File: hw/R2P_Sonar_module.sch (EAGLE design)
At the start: 36 parts, among them U1 STM32F103CX, U5 LD3985XX, X1 MICROMATCH-4, X2 MICROMATCH-6, X3 MICROMATCH-6-SIDE

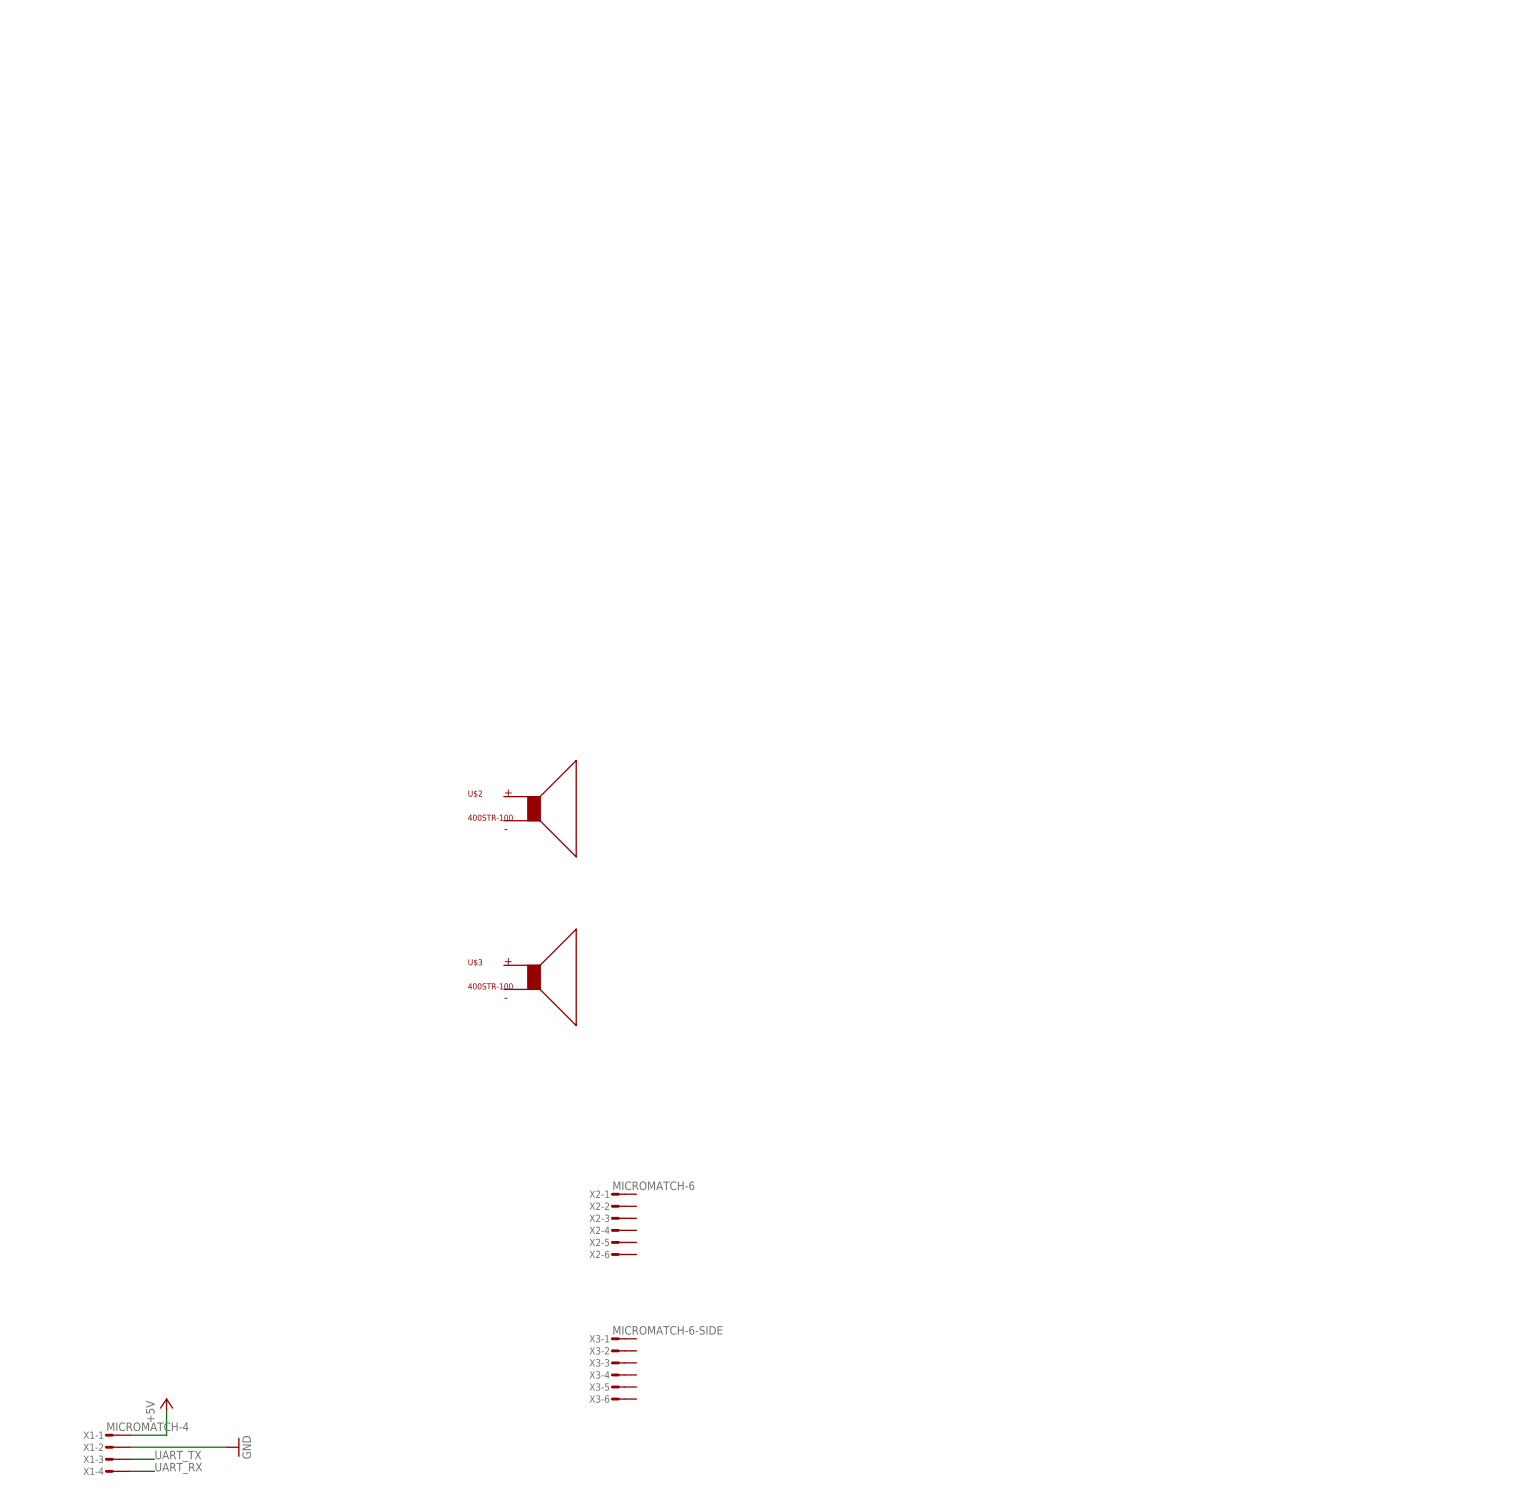
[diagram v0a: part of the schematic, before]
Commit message: Ongoing layout
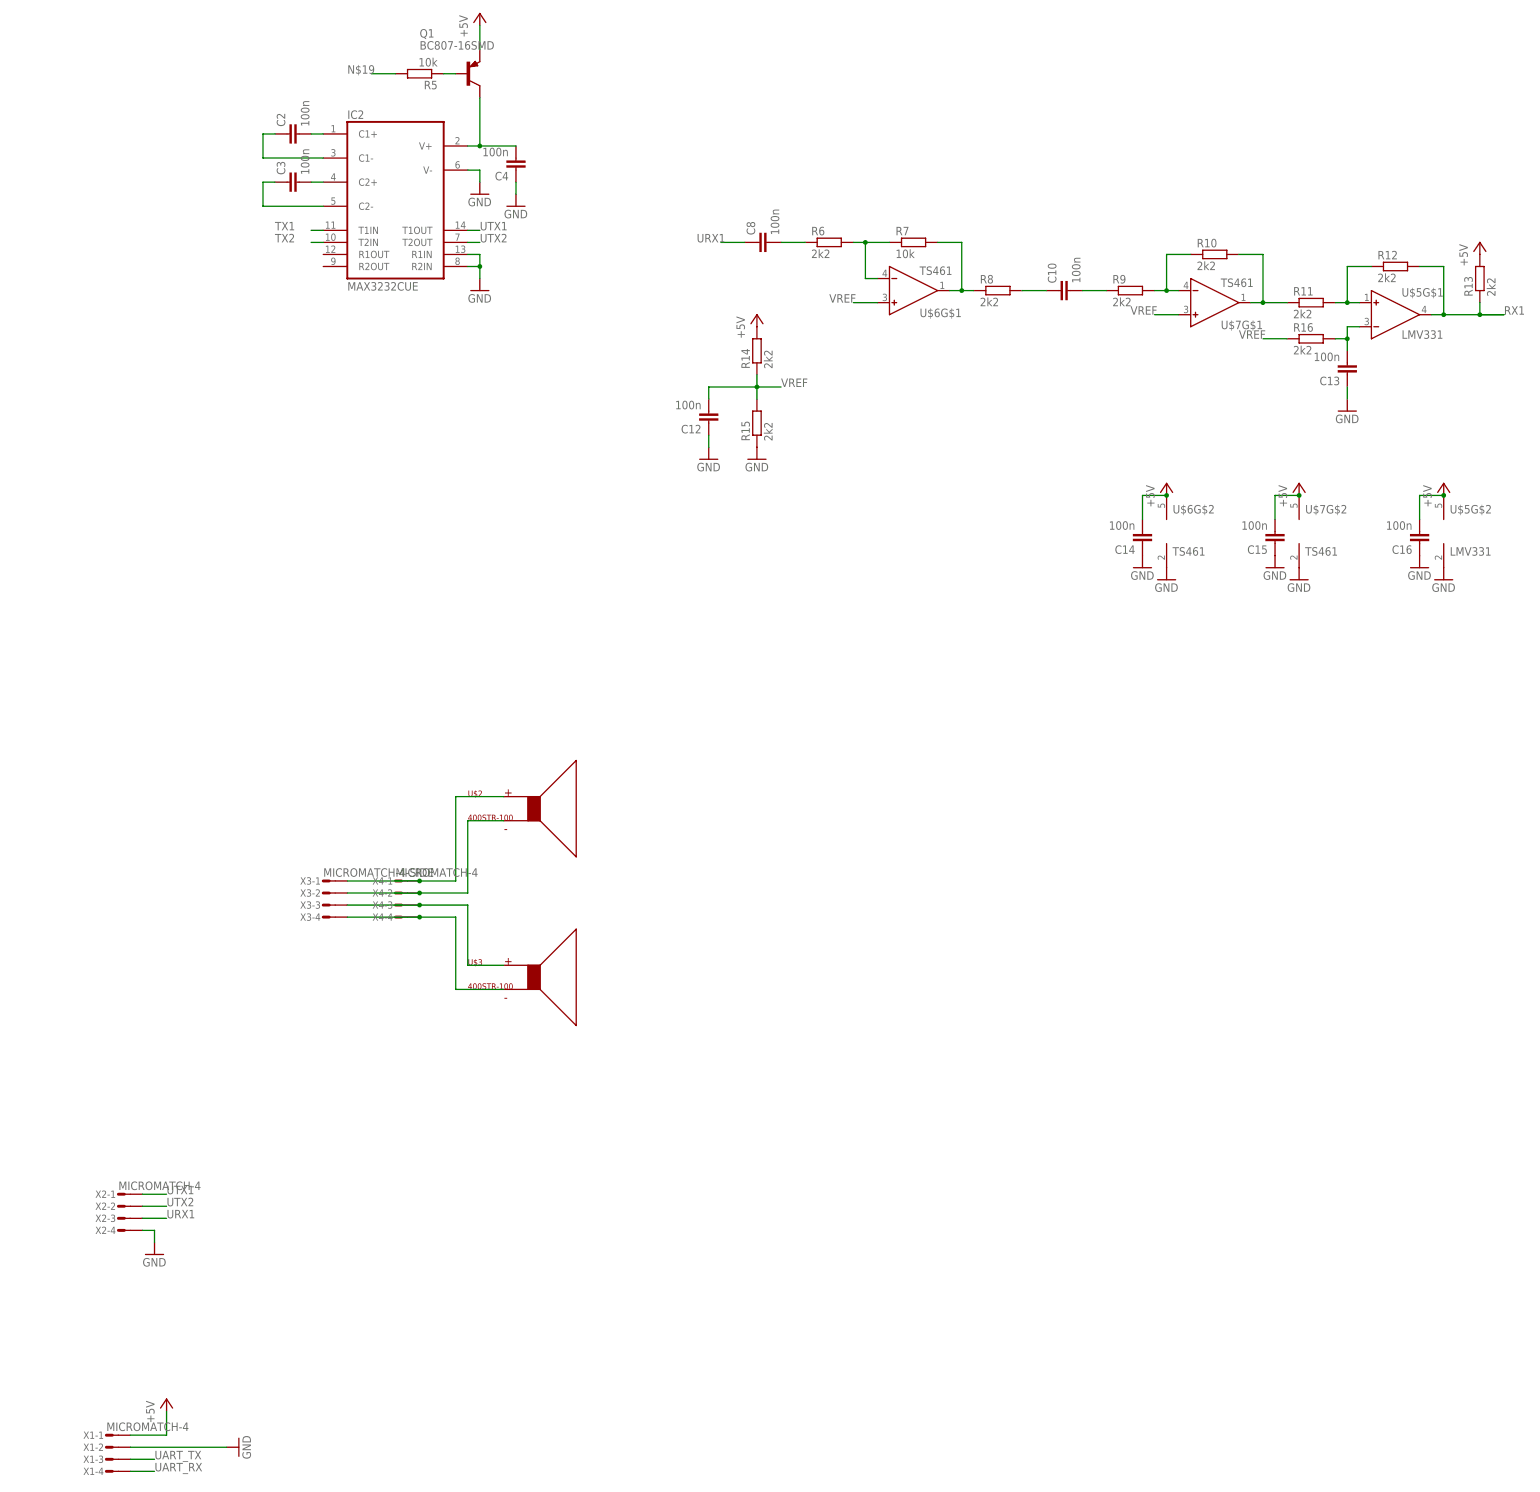
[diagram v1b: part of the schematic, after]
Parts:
- added C10, C12, C13, C14, C15, C16, C2, C3, C4, C8: 100n, rcl:C-EUC0603
- added IC2: MAX3232CUE, maxim:MAX3232CUE
- added Q1: BC807-16SMD, transistor-pnp:BC807-16SMD
- added R10, R11, R12, R13, R14, R15, R16, R6, R8, R9: 2k2, rcl:R-EU_R0603
- added R5, R7: 10k, rcl:R-EU_R0603
- added U$5: LMV331, texas-instruments:LMV331
- added U$6, U$7: TS461, st:TS461
- added X4: MICROMATCH-4, tyco:MICROMATCH-4
- X2: value MICROMATCH-6 -> MICROMATCH-4; device tyco:MICROMATCH-6 -> tyco:MICROMATCH-4
- X3: value MICROMATCH-6-SIDE -> MICROMATCH-4-SIDE; device tyco:MICROMATCH-6-SIDE -> apbteam_con-amp-micromatch:MICROMATCH-4-SIDE
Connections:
- new net N$10: C4.2, IC2G$1.V+, Q1.C
- new net N$11: C8.2, R6.1
- new net N$12: U$2.P$1, X3-1.S, X4-1.S
- new net N$13: U$2.P$2, X3-2.S, X4-2.S
- new net N$14: U$3.P$1, X3-3.S, X4-3.S
- new net N$16: U$3.P$2, X3-4.S, X4-4.S
- new net N$17: Q1.B, R5.1
- new net N$19: R5.2
- new net N$21: R6.2, R7.1, U$6G$1.IN-
- new net N$23: R7.2, R8.1, U$6G$1.OUT
- new net N$24: C10.1, R8.2
- new net N$25: C10.2, R9.1
- new net N$26: R10.1, R9.2, U$7G$1.IN-
- new net N$27: R10.2, R11.1, U$7G$1.OUT
- new net N$28: R11.2, R12.1, U$5G$1.IN+
- new net N$30: C13.2, R16.2, U$5G$1.IN-
- new net N$6: C2.2, IC2G$1.C1+
- new net N$7: C2.1, IC2G$1.C1-
- new net N$8: C3.2, IC2G$1.C2+
- new net N$9: C3.1, IC2G$1.C2-
- new net RX1: R12.2, R13.1, U$5G$1.OUT
- new net TX1: IC2G$1.T1IN
- new net TX2: IC2G$1.T2IN
- new net URX1: C8.1, X2-3.S
- new net UTX1: IC2G$1.T1OUT, X2-1.S
- new net UTX2: IC2G$1.T2OUT, X2-2.S
- new net VREF: C12.2, R14.1, R15.2, R16.1, U$6G$1.IN+, U$7G$1.IN+
- net +5V: now also C14.2, C15.2, C16.2, Q1.E, R13.2, R14.2, U$5G$2.V+, U$6G$2.V+, U$7G$2.V+
- net GND: now also C12.1, C13.1, C14.1, C15.1, C16.1, C4.1, IC2G$1.R1IN, IC2G$1.R2IN, IC2G$1.V-, R15.1, U$5G$2.V-, U$6G$2.V-, U$7G$2.V-, X2-4.S
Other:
- moved on the sheet: X2-1, X2-2, X2-3, X2-4, X3-1, X3-2, X3-3, X3-4
